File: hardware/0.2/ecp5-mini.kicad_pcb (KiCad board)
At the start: 4 copper layers, 52 x 27 mm, 112 parts, among them J1 Micro_SD_Card, J2 JTAG, J3 S7 Mini, J4 S7 Mini, J5 USB_Type_C_2.0, Q500 BSS138, Q501 BSS138, Q502 BSS138, Q503 BSS138, SW1 PTS810, U1 W25Q128JVPIQ, U2 ECP5U_12_CABGA256, U3 S27KS0641, U4 TLV75525PDQNR, U5 TLV75518PDQNR, U6 USBLC6-2P6, U7 TLV62569DRLR, U8 TLV62569DRLR, X1 16MHz

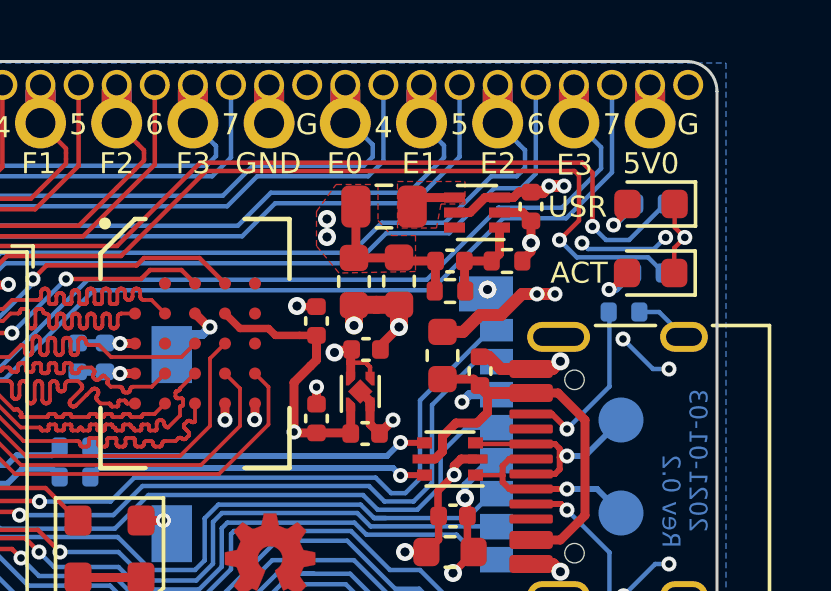
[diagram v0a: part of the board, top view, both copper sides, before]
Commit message: post 0.2 assembly updates
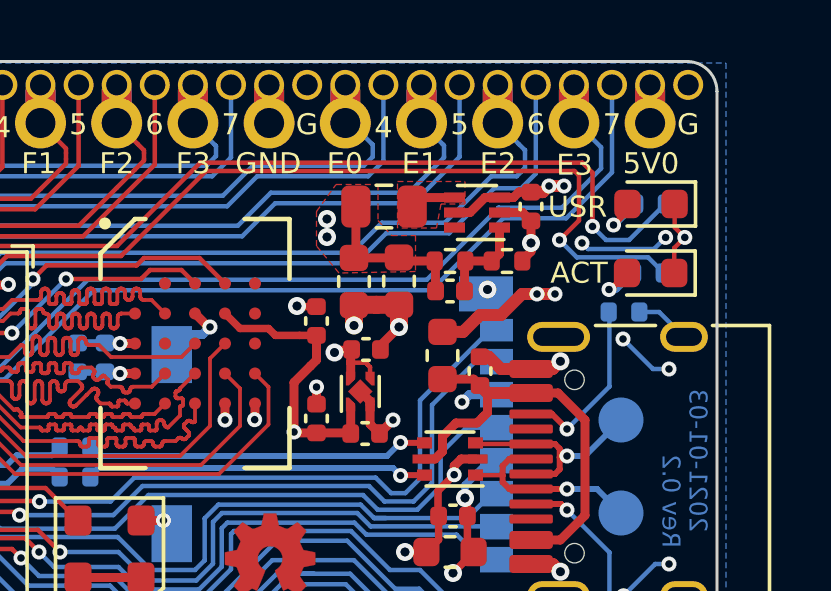
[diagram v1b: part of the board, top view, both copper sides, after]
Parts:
- moved C14 1.00 mm to (139.3, 89.1)
- moved R2 1.00 mm to (139.3, 88.1)

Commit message: nightly version bump
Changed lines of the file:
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@@
-(kicad_pcb (version 20210126) (generator pcbnew)
+(kicad_pcb (version 20210228) (generator pcbnew)
   (general
     (thickness 1.6)
@@
       (dielectric_constraints no)
     )
+    (pad_to_mask_clearance 0)
     (pcbplotparams
       (layerselection 0x00010fc_ffffffff)
@@
     (fp_line (start 3 -2.5) (end 3 2.5) (layer "F.Fab") (width 0.1))
     (fp_line (start -3 -1.5) (end -2 -2.5) (layer "F.Fab") (width 0.1))
-    (pad "" smd roundrect (at -0.85 -1.075 270) (locked) (size 1.37 1.73) (layers "F.Paste") (roundrect_rratio 0.1824817518248175))
-    (pad "" smd roundrect (at -0.85 1.075 270) (locked) (size 1.37 1.73) (layers "F.Paste") (roundrect_rratio 0.1824817518248175))
-    (pad "" smd roundrect (at 0.85 -1.075 270) (locked) (size 1.37 1.73) (layers "F.Paste") (roundrect_rratio 0.1824817518248175))
-    (pad "" smd roundrect (at 0.85 1.075 270) (locked) (size 1.37 1.73) (layers "F.Paste") (roundrect_rratio 0.1824817518248175))
+    (pad "" smd roundrect (at -0.85 -1.075 270) (locked) (size 1.37 1.73) (layers "F.Paste") (roundrect_rratio 0.1824817518))
+    (pad "" smd roundrect (at -0.85 1.075 270) (locked) (size 1.37 1.73) (layers "F.Paste") (roundrect_rratio 0.1824817518))
+    (pad "" smd roundrect (at 0.85 -1.075 270) (locked) (size 1.37 1.73) (layers "F.Paste") (roundrect_rratio 0.1824817518))
+    (pad "" smd roundrect (at 0.85 1.075 270) (locked) (size 1.37 1.73) (layers "F.Paste") (roundrect_rratio 0.1824817518))
     (pad "1" smd roundrect (at -2.7 -1.905 270) (locked) (size 0.75 0.5) (layers "F.Cu" "F.Paste" "F.Mask") (roundrect_rratio 0.25)
       (net 68 "/FPGA Config/CFG_CS") (pinfunction "~CS"))
@@
     (pad "8" smd roundrect (at 2.7 -1.905 270) (locked) (size 0.75 0.5) (layers "F.Cu" "F.Paste" "F.Mask") (roundrect_rratio 0.25)
       (net 53 "+3V3") (pinfunction "VCC"))
-    (pad "9" smd roundrect (at 0 0 270) (locked) (size 3.4 4.3) (layers "F.Cu" "F.Mask") (roundrect_rratio 0.07352911764705883)
+    (pad "9" smd roundrect (at 0 0 270) (locked) (size 3.4 4.3) (layers "F.Cu" "F.Mask") (roundrect_rratio 0.07352911765)
       (net 41 "GND") (pinfunction "GND"))
     (model "${KISYS3DMOD}/Package_DFN_QFN.3dshapes/DFN-8-1EP_6x5mm_P1.27mm_EP4x4mm.step"
